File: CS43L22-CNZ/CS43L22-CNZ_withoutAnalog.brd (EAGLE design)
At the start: 39.8 x 28 mm, 35 parts, among them IC1 CS43L22-CNZ, IC2 LP3985IM5-2.5, J2 1503_02

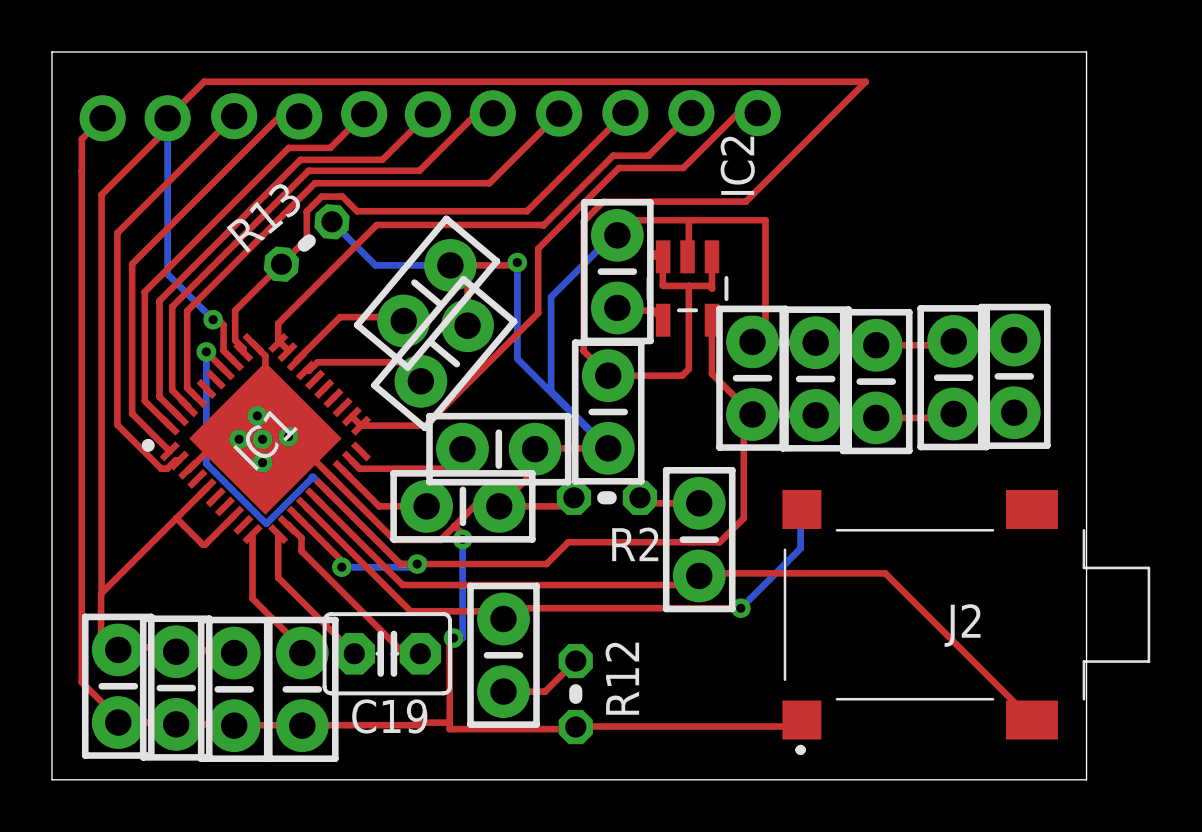
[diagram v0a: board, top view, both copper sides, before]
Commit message: added final
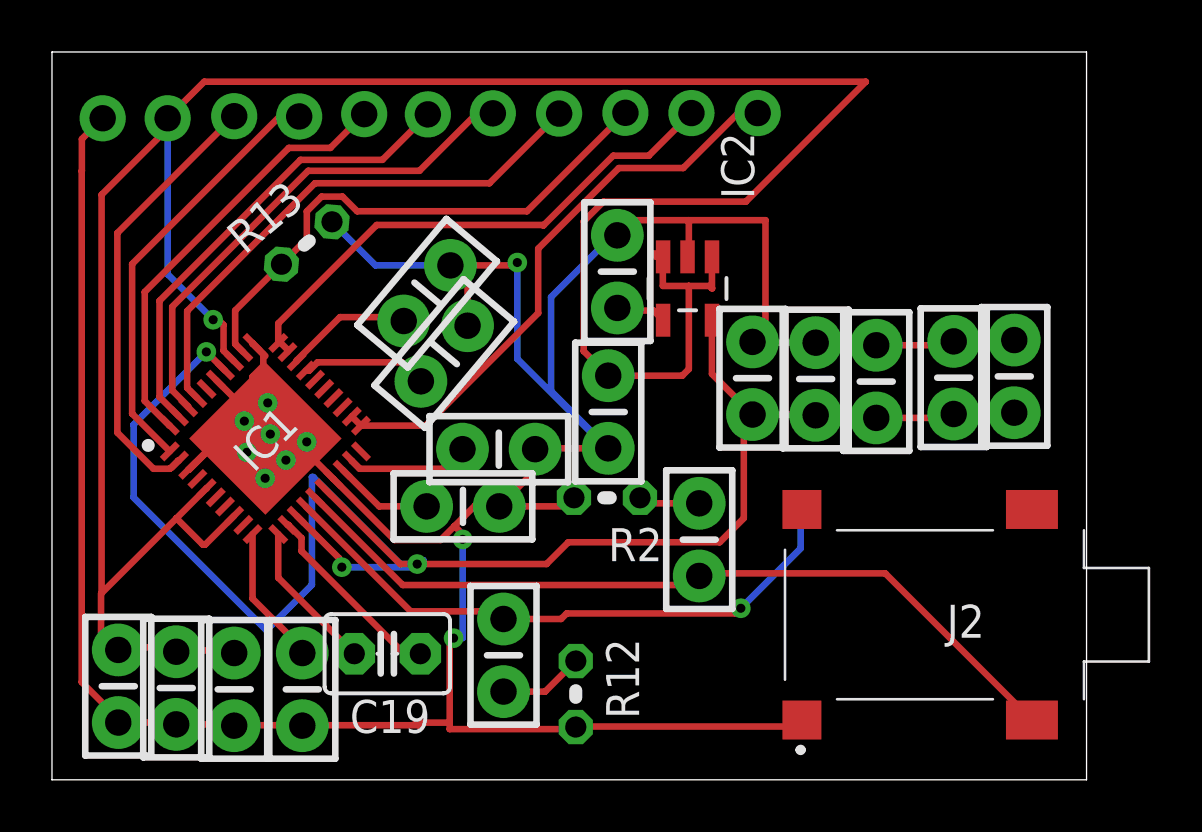
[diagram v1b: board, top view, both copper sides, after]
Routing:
- net N$23: track 15.2 -> 0.00 mm
- net N$22: track 10.6 -> 0.00 mm
- net 2.5V: track 60.0 -> 70.5 mm
- net GND: track 139.0 -> 144.4 mm
- net N$21: track 1.55 -> 0.00 mm
- net N$12: track 1.20 -> 0.00 mm
- net N$20: track 0.92 -> 0.00 mm
- added copper zone on layer 16, net HEAT
- removed copper zone on layer 16, net GND
